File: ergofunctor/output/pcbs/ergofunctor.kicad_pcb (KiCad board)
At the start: 2 copper layers, 155.9 x 135.1 mm, 56 parts

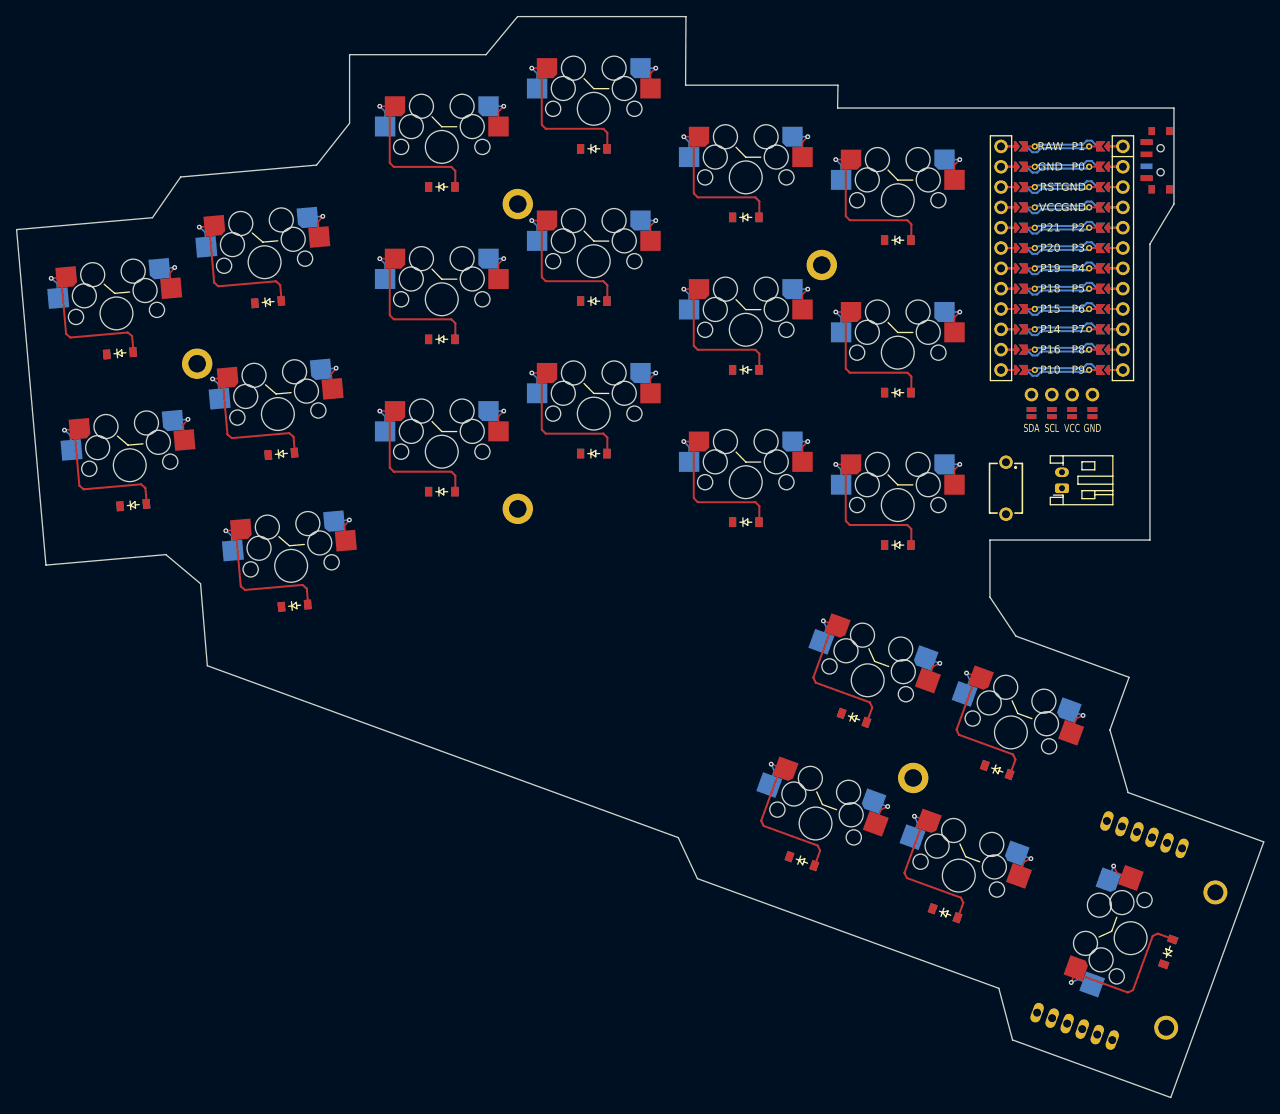
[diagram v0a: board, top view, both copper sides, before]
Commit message: fix joystick
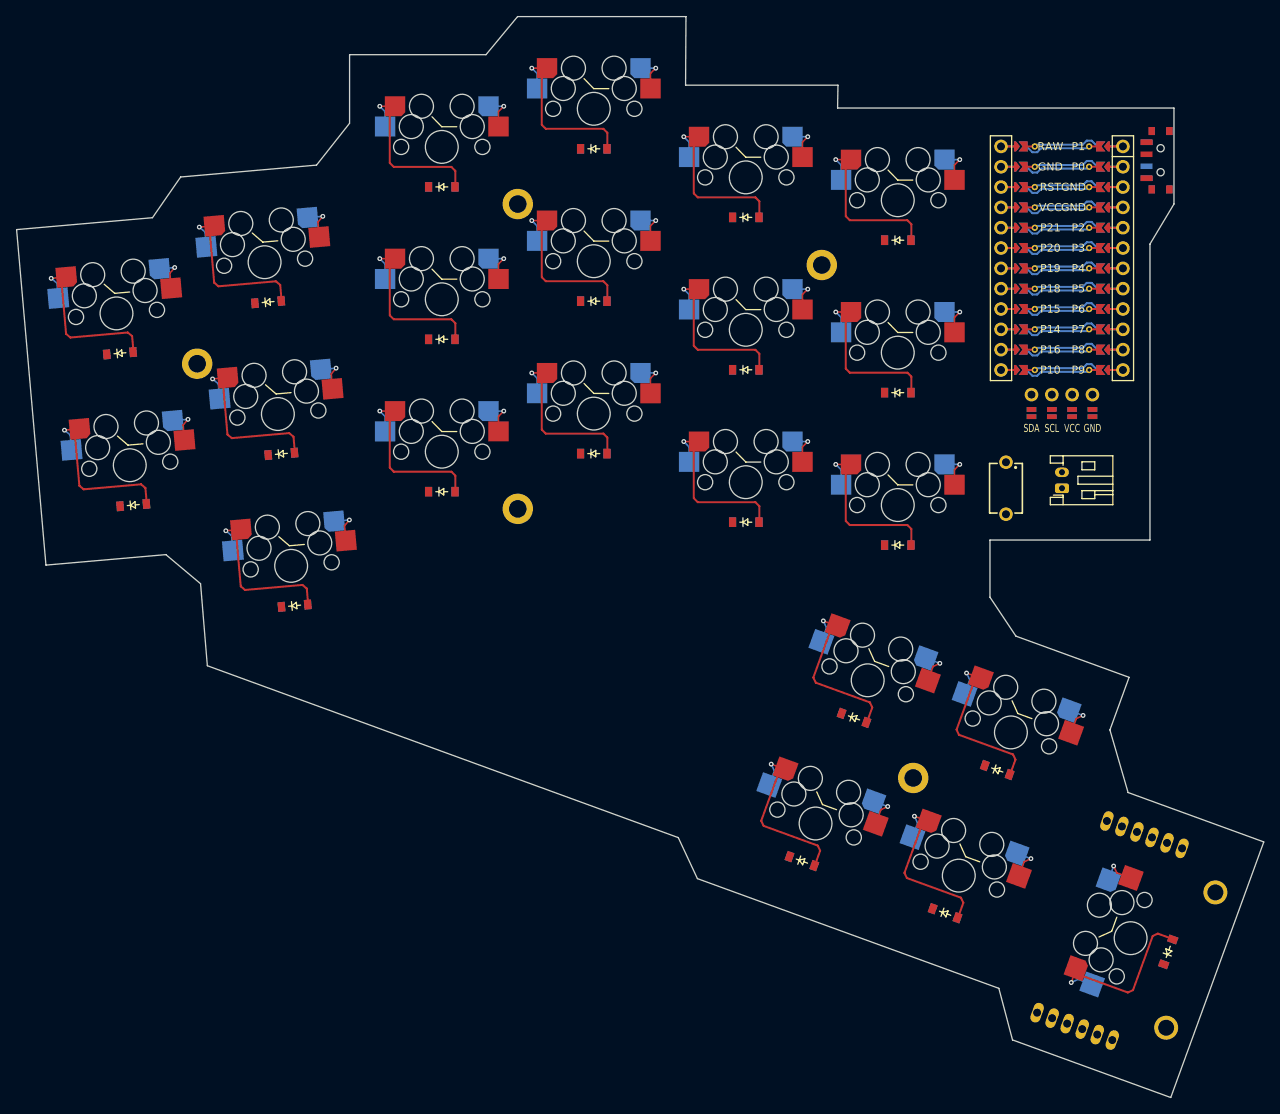
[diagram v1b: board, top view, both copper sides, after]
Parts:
- _23: moved to F.Cu
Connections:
- S1 pad 1: outer_home -> P4
- S10 pad 1: middle_home -> P7
- S11 pad 1: middle_top -> P7
- S12 pad 1: index_bottom -> P8
- S13 pad 1: index_home -> P8
- S14 pad 1: index_top -> P8
- S15 pad 1: inner_bottom -> P9
- S16 pad 1: inner_home -> P9
- S17 pad 1: inner_top -> P9
- S18 pad 1: outer_top_row -> P4
- S19 pad 1: middle_top_row -> P5
- S2 pad 1: outer_top -> P4
- S20 pad 1: outer_bottom_row -> P6
- S21 pad 1: middle_bottom_row -> P7
- S22 pad 1: inner_row -> P8
- S3 pad 1: innerp_bottom -> P5
- S4 pad 1: innerp_home -> P5
- S5 pad 1: innerp_top -> P5
- S6 pad 1: ring_bottom -> P6
- S7 pad 1: ring_home -> P6
- S8 pad 1: ring_top -> P6
- S9 pad 1: middle_bottom -> P7
- XX1 pad 5: inner_rowb -> inner_row
- XX2 pad 5: inner_rowb -> inner_row
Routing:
- net (no net): track 731.1 -> 0.00 mm
- net GND: track 0.00 -> 29.5 mm
- net middle_bottom_row: track 4.72 -> 22.6 mm
- net outer_top_row: track 4.72 -> 22.6 mm
- net inner_row: track 4.72 -> 22.6 mm
- net innerp_top: track 4.72 -> 22.6 mm
- net innerp_home: track 4.72 -> 22.6 mm
- net outer_home: track 4.72 -> 22.6 mm
- net outer_top: track 4.72 -> 22.6 mm
- net ring_bottom: track 4.72 -> 22.6 mm
- net index_bottom: track 4.72 -> 22.6 mm
- net middle_top: track 4.72 -> 22.6 mm
- net middle_bottom: track 4.72 -> 22.6 mm
- net ring_top: track 4.72 -> 22.6 mm
- net middle_home: track 4.72 -> 22.6 mm
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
